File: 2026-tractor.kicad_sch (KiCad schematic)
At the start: 8 parts, among them K1 Fujitsu_FTR-LYAA005x, SW1 SW_Nidec_CAS-120A1, U1 4060

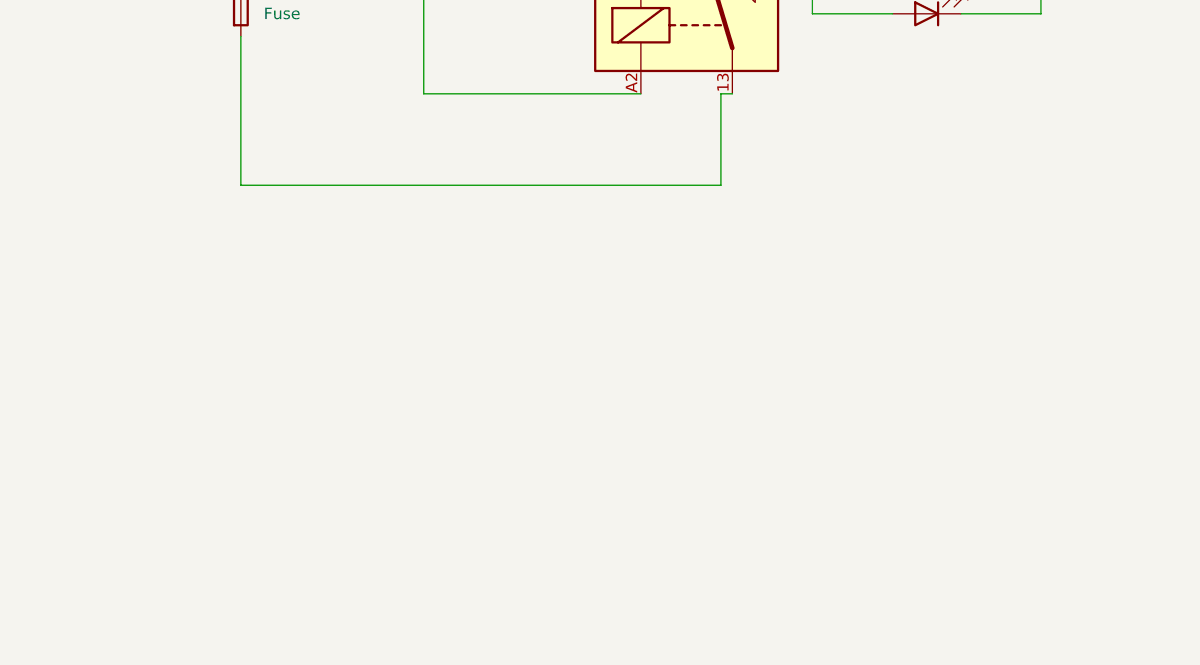
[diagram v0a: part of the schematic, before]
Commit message: Lighitng Schematic completed
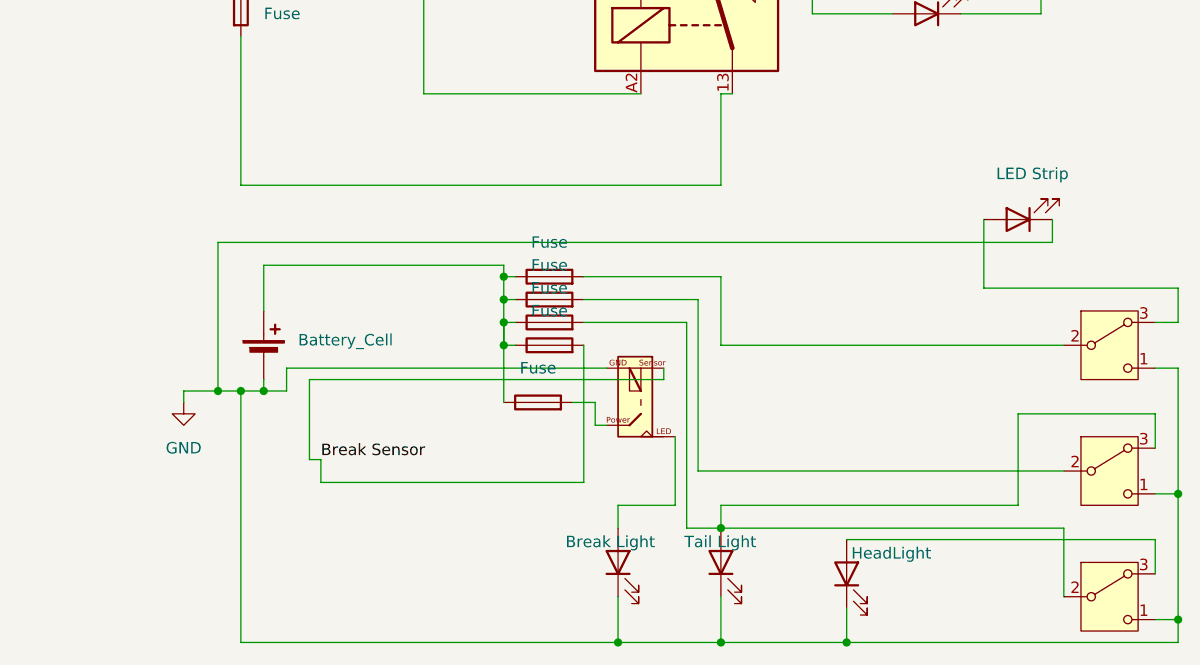
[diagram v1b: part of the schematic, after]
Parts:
- added BT2: Battery_Cell, symbol Device:Battery_Cell
- added D3: LED Strip, symbol Device:LED
- added D4: Break Light, symbol Device:LED
- added D5: Tail Light, symbol Device:LED
- added D6: HeadLight, symbol Device:LED
- added F3, F4, F5, F6, F7: Fuse, symbol Device:Fuse
- added K2: Fujitsu_FTR-LYAA005x, Relay_THT:Relay_SPST-NO_Fujitsu_FTR-LYAA005x_FormA_Vertical, symbol Relay:Fujitsu_FTR-LYAA005x
- added SW2, SW3, SW4: SW_Nidec_CAS-120A1, Button_Switch_SMD:Nidec_Copal_CAS-120A, symbol Switch:SW_Nidec_CAS-120A1
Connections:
- net GND: now also BT2.2 (-), D3.1 (K), D4.1 (K), D5.1 (K), D6.1 (K), K2.GND, SW2.1 (C), SW3.1 (C), SW4.1 (C)
- new net: BT2.1 (+), F3.1, F4.1, F5.1, F6.1, F7.1
- new net: D3.2 (A), SW4.3 (A)
- new net: F3.2, SW4.2 (B)
- new net: D6.2 (A), SW2.3 (A)
- new net: D5.2 (A), F5.2, SW2.2 (B), SW3.3 (A)
- new net: F7.2, K2.Power
- new net: D4.2 (A), K2.LED
- new net: F4.2, SW3.2 (B)
- new net Break Sensor: F6.2, K2.Sensor
